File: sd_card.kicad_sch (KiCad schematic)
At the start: 2 parts, among them J2 Micro_SD_Card

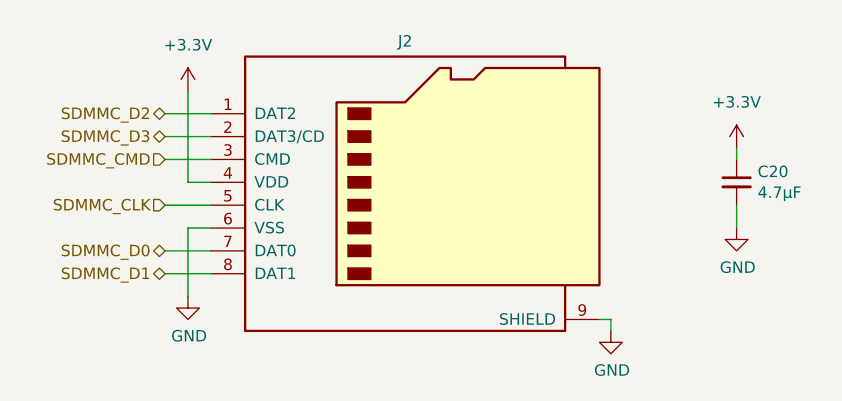
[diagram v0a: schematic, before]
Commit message: Assign footprints to symbols
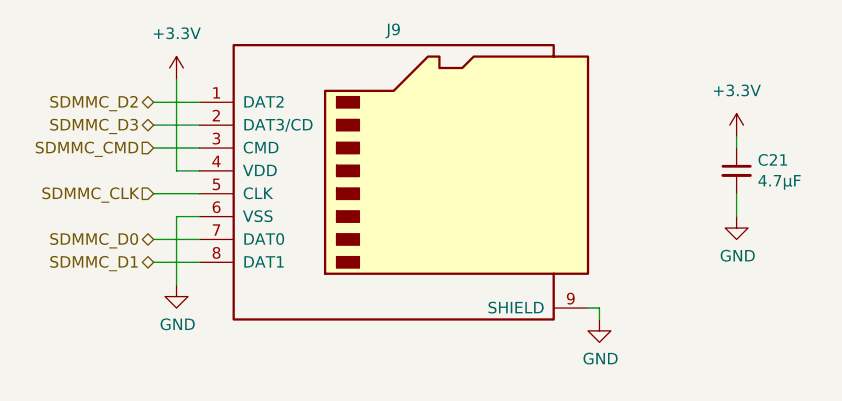
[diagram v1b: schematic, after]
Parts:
- J9: renamed from J2; footprint PUTM_Kicad_FOOTPRINTS:112K-TAA0-RA1 -> Local_Library:112K-TAA0-RA1
- renumbered C20 to C21
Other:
- moved on the sheet: C21, J9
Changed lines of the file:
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@@
     (title "SD Card")
     (date "2022-12-17")
-    (rev "0.1.0")
+    (rev "${REVISION}")
   )
-  (wire (pts (xy 176.53 116.84) (xy 175.26 116.84))
+  (wire (pts (xy 175.26 115.57) (xy 173.99 115.57))
     (stroke (width 0) (type default) (color 0 0 0 0))
   )
-  (wire (pts (xy 127 93.98) (xy 132.08 93.98))
+  (wire (pts (xy 125.73 92.71) (xy 130.81 92.71))
     (stroke (width 0) (type default) (color 0 0 0 0))
   )
-  (wire (pts (xy 132.08 111.76) (xy 127 111.76))
+  (wire (pts (xy 130.81 110.49) (xy 125.73 110.49))
     (stroke (width 0) (type default) (color 0 0 0 0))
   )
-  (wire (pts (xy 127 104.14) (xy 132.08 104.14))
+  (wire (pts (xy 125.73 102.87) (xy 130.81 102.87))
     (stroke (width 0) (type default) (color 0 0 0 0))
   )
-  (wire (pts (xy 129.54 106.68) (xy 132.08 106.68))
+  (wire (pts (xy 128.27 105.41) (xy 130.81 105.41))
     (stroke (width 0) (type default) (color 0 0 0 0))
   )
-  (wire (pts (xy 190.5 104.14) (xy 190.5 106.68))
+  (wire (pts (xy 190.5 102.87) (xy 190.5 105.41))
     (stroke (width 0) (type default) (color 0 0 0 0))
   )
-  (wire (pts (xy 176.53 118.11) (xy 176.53 116.84))
+  (wire (pts (xy 175.26 116.84) (xy 175.26 115.57))
     (stroke (width 0) (type default) (color 0 0 0 0))
   )
-  (wire (pts (xy 127 96.52) (xy 132.08 96.52))
+  (wire (pts (xy 125.73 95.25) (xy 130.81 95.25))
     (stroke (width 0) (type default) (color 0 0 0 0))
   )
-  (wire (pts (xy 127 109.22) (xy 132.08 109.22))
+  (wire (pts (xy 125.73 107.95) (xy 130.81 107.95))
     (stroke (width 0) (type default) (color 0 0 0 0))
   )
-  (wire (pts (xy 190.5 97.79) (xy 190.5 99.06))
+  (wire (pts (xy 190.5 96.52) (xy 190.5 97.79))
     (stroke (width 0) (type default) (color 0 0 0 0))
   )
-  (wire (pts (xy 132.08 101.6) (xy 129.54 101.6))
+  (wire (pts (xy 130.81 100.33) (xy 128.27 100.33))
     (stroke (width 0) (type default) (color 0 0 0 0))
   )
-  (wire (pts (xy 129.54 114.3) (xy 129.54 106.68))
+  (wire (pts (xy 128.27 113.03) (xy 128.27 105.41))
     (stroke (width 0) (type default) (color 0 0 0 0))
   )
-  (wire (pts (xy 129.54 91.44) (xy 129.54 101.6))
+  (wire (pts (xy 128.27 90.17) (xy 128.27 100.33))
     (stroke (width 0) (type default) (color 0 0 0 0))
   )
-  (wire (pts (xy 127 99.06) (xy 132.08 99.06))
+  (wire (pts (xy 125.73 97.79) (xy 130.81 97.79))
     (stroke (width 0) (type default) (color 0 0 0 0))
   )
-  (hierarchical_label "SDMMC_D3" (shape bidirectional) (at 127 96.52 180)
+  (hierarchical_label "SDMMC_D3" (shape bidirectional) (at 125.73 95.25 180)
     (effects (font (size 1.27 1.27)) (justify right))
   )
-  (hierarchical_label "SDMMC_D1" (shape bidirectional) (at 127 111.76 180)
+  (hierarchical_label "SDMMC_D1" (shape bidirectional) (at 125.73 110.49 180)
     (effects (font (size 1.27 1.27)) (justify right))
   )
-  (hierarchical_label "SDMMC_D2" (shape bidirectional) (at 127 93.98 180)
+  (hierarchical_label "SDMMC_D2" (shape bidirectional) (at 125.73 92.71 180)
     (effects (font (size 1.27 1.27)) (justify right))
   )
-  (hierarchical_label "SDMMC_D0" (shape bidirectional) (at 127 109.22 180)
+  (hierarchical_label "SDMMC_D0" (shape bidirectional) (at 125.73 107.95 180)
     (effects (font (size 1.27 1.27)) (justify right))
   )
-  (hierarchical_label "SDMMC_CLK" (shape input) (at 127 104.14 180)
+  (hierarchical_label "SDMMC_CLK" (shape input) (at 125.73 102.87 180)
     (effects (font (size 1.27 1.27)) (justify right))
   )
-  (hierarchical_label "SDMMC_CMD" (shape input) (at 127 99.06 180)
+  (hierarchical_label "SDMMC_CMD" (shape input) (at 125.73 97.79 180)
     (effects (font (size 1.27 1.27)) (justify right))
   )
-  (symbol (lib_id "Connector:Micro_SD_Card") (at 154.94 101.6 0) (unit 1)
+  (symbol (lib_id "Connector:Micro_SD_Card") (at 153.67 100.33 0) (unit 1)
     (in_bom yes) (on_board yes)
-    (property "Reference" "J2" (id 0) (at 153.67 85.9282 0))
-    (property "Value" "Micro_SD_Card" (id 1) (at 153.67 85.6996 0)
+    (property "Reference" "J9" (id 0) (at 152.4 84.6582 0))
+    (property "Value" "Micro_SD_Card" (id 1) (at 152.4 84.4296 0)
       (effects (font (size 1.27 1.27)) hide)
     )
-    (property "Footprint" "PUTM_Kicad_FOOTPRINTS:112K-TAA0-RA1" (id 2) (at 184.15 93.98 0)
+    (property "Footprint" "Local_Library:112K-TAA0-RA1" (id 2) (at 182.88 92.71 0)
       (effects (font (size 1.27 1.27)) hide)
     )
-    (property "Datasheet" "https://www.tme.eu/Document/c3b9a7ded342d5553aff6a91c42e4fab/112K-TAA0-RA1.pdf" (id 3) (at 154.94 101.6 0)
+    (property "Datasheet" "https://www.tme.eu/Document/c3b9a7ded342d5553aff6a91c42e4fab/112K-TAA0-RA1.pdf" (id 3) (at 153.67 100.33 0)
       (effects (font (size 1.27 1.27)) hide)
     )
@@
     (pin "9")
   )
-  (symbol (lib_id "Device:C_Small") (at 190.5 101.6 0) (unit 1)
+  (symbol (lib_id "Device:C_Small") (at 190.5 100.33 0) (unit 1)
     (in_bom yes) (on_board yes)
-    (property "Reference" "C20" (id 0) (at 192.8368 100.4316 0)
+    (property "Reference" "C21" (id 0) (at 192.8368 99.1616 0)
       (effects (font (size 1.27 1.27)) (justify left))
     )
-    (property "Value" "4.7μF" (id 1) (at 192.8368 102.743 0)
+    (property "Value" "4.7μF" (id 1) (at 192.8368 101.473 0)
       (effects (font (size 1.27 1.27)) (justify left))
     )
-    (property "Footprint" "Capacitor_SMD:C_0603_1608Metric" (id 2) (at 190.5 101.6 0)
+    (property "Footprint" "Capacitor_SMD:C_0603_1608Metric" (id 2) (at 190.5 100.33 0)
       (effects (font (size 1.27 1.27)) hide)
     )
-    (property "Datasheet" "~" (id 3) (at 190.5 101.6 0)
+    (property "Datasheet" "~" (id 3) (at 190.5 100.33 0)
       (effects (font (size 1.27 1.27)) hide)
     )
-    (property "LCSC" "C19666" (id 4) (at 190.5 101.6 0)
+    (property "LCSC" "C19666" (id 4) (at 190.5 100.33 0)
       (effects (font (size 1.27 1.27)) hide)
     )
@@
     (pin "2")
   )
-  (symbol (lib_id "power:GND") (at 190.5 106.68 0) (unit 1)
+  (symbol (lib_id "power:GND") (at 190.5 105.41 0) (unit 1)
     (in_bom yes) (on_board yes)
-    (property "Reference" "#PWR040" (id 0) (at 190.5 113.03 0)
+    (property "Reference" "#PWR053" (id 0) (at 190.5 111.76 0)
       (effects (font (size 1.27 1.27)) hide)
     )
-    (property "Value" "GND" (id 1) (at 190.627 111.0742 0))
-    (property "Footprint" "" (id 2) (at 190.5 106.68 0)
+    (property "Value" "GND" (id 1) (at 190.627 109.8042 0))
+    (property "Footprint" "" (id 2) (at 190.5 105.41 0)
       (effects (font (size 1.27 1.27)) hide)
     )
-    (property "Datasheet" "" (id 3) (at 190.5 106.68 0)
+    (property "Datasheet" "" (id 3) (at 190.5 105.41 0)
       (effects (font (size 1.27 1.27)) hide)
     )
     (pin "1")
   )
-  (symbol (lib_id "power:+3.3V") (at 190.5 97.79 0) (unit 1)
+  (symbol (lib_id "power:+3.3V") (at 190.5 96.52 0) (unit 1)
     (in_bom yes) (on_board yes) (fields_autoplaced)
-    (property "Reference" "#PWR039" (id 0) (at 190.5 101.6 0)
+    (property "Reference" "#PWR052" (id 0) (at 190.5 100.33 0)
       (effects (font (size 1.27 1.27)) hide)
     )
-    (property "Value" "+3.3V" (id 1) (at 190.5 92.71 0))
-    (property "Footprint" "" (id 2) (at 190.5 97.79 0)
+    (property "Value" "+3.3V" (id 1) (at 190.5 91.44 0))
+    (property "Footprint" "" (id 2) (at 190.5 96.52 0)
       (effects (font (size 1.27 1.27)) hide)
     )
-    (property "Datasheet" "" (id 3) (at 190.5 97.79 0)
+    (property "Datasheet" "" (id 3) (at 190.5 96.52 0)
       (effects (font (size 1.27 1.27)) hide)
     )
     (pin "1")
   )
-  (symbol (lib_id "power:+3.3V") (at 129.54 91.44 0) (unit 1)
+  (symbol (lib_id "power:+3.3V") (at 128.27 90.17 0) (unit 1)
     (in_bom yes) (on_board yes) (fields_autoplaced)
-    (property "Reference" "#PWR038" (id 0) (at 129.54 95.25 0)
+    (property "Reference" "#PWR051" (id 0) (at 128.27 93.98 0)
       (effects (font (size 1.27 1.27)) hide)
     )
-    (property "Value" "+3.3V" (id 1) (at 129.54 86.36 0))
-    (property "Footprint" "" (id 2) (at 129.54 91.44 0)
+    (property "Value" "+3.3V" (id 1) (at 128.27 85.09 0))
+    (property "Footprint" "" (id 2) (at 128.27 90.17 0)
       (effects (font (size 1.27 1.27)) hide)
     )
-    (property "Datasheet" "" (id 3) (at 129.54 91.44 0)
+    (property "Datasheet" "" (id 3) (at 128.27 90.17 0)
       (effects (font (size 1.27 1.27)) hide)
     )
     (pin "1")
   )
-  (symbol (lib_id "power:GND") (at 129.54 114.3 0) (unit 1)
+  (symbol (lib_id "power:GND") (at 128.27 113.03 0) (unit 1)
     (in_bom yes) (on_board yes)
-    (property "Reference" "#PWR041" (id 0) (at 129.54 120.65 0)
+    (property "Reference" "#PWR054" (id 0) (at 128.27 119.38 0)
       (effects (font (size 1.27 1.27)) hide)
     )
-    (property "Value" "GND" (id 1) (at 129.667 118.6942 0))
-    (property "Footprint" "" (id 2) (at 129.54 114.3 0)
+    (property "Value" "GND" (id 1) (at 128.397 117.4242 0))
+    (property "Footprint" "" (id 2) (at 128.27 113.03 0)
       (effects (font (size 1.27 1.27)) hide)
     )
-    (property "Datasheet" "" (id 3) (at 129.54 114.3 0)
+    (property "Datasheet" "" (id 3) (at 128.27 113.03 0)
       (effects (font (size 1.27 1.27)) hide)
     )
     (pin "1")
   )
-  (symbol (lib_id "power:GND") (at 176.53 118.11 0) (unit 1)
+  (symbol (lib_id "power:GND") (at 175.26 116.84 0) (unit 1)
     (in_bom yes) (on_board yes)
-    (property "Reference" "#PWR042" (id 0) (at 176.53 124.46 0)
+    (property "Reference" "#PWR055" (id 0) (at 175.26 123.19 0)
       (effects (font (size 1.27 1.27)) hide)
     )
-    (property "Value" "GND" (id 1) (at 176.657 122.5042 0))
-    (property "Footprint" "" (id 2) (at 176.53 118.11 0)
+    (property "Value" "GND" (id 1) (at 175.387 121.2342 0))
+    (property "Footprint" "" (id 2) (at 175.26 116.84 0)
       (effects (font (size 1.27 1.27)) hide)
     )
-    (property "Datasheet" "" (id 3) (at 176.53 118.11 0)
+    (property "Datasheet" "" (id 3) (at 175.26 116.84 0)
       (effects (font (size 1.27 1.27)) hide)
     )
